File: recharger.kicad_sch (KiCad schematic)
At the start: 20 parts, among them J1 Battery Connector, U2 BQ25887RGE

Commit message: update PCB
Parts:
- J1: footprint Connector_JST:JST_PH_S4B-PH-K_1x04_P2.00mm_Horizontal -> Connector_JST:JST_PH_S4B-PH-SM4-TB_1x04-1MP_P2.00mm_Horizontal
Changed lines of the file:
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@@
 			)
 		)
-		(property "Footprint" "Connector_JST:JST_PH_S4B-PH-K_1x04_P2.00mm_Horizontal"
+		(property "Footprint" "Connector_JST:JST_PH_S4B-PH-SM4-TB_1x04-1MP_P2.00mm_Horizontal"
 			(at 194.31 110.49 0)
 			(hide yes)

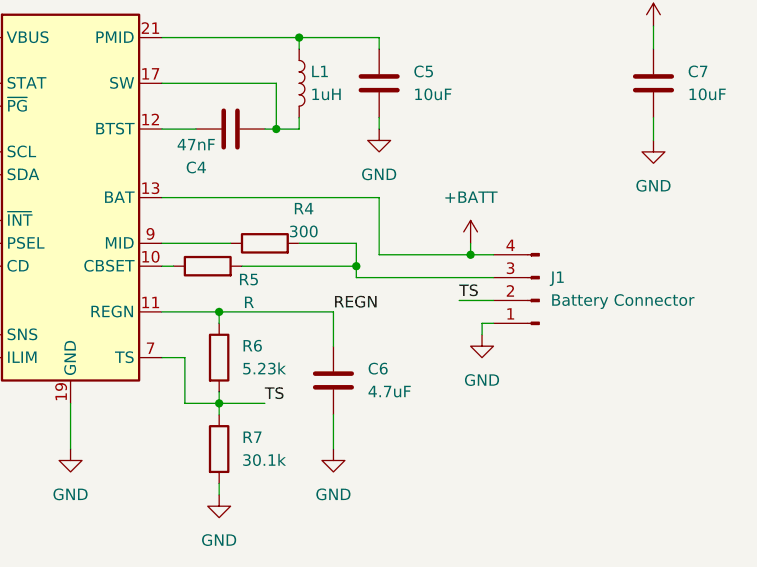
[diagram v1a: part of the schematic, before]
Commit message: more on layout
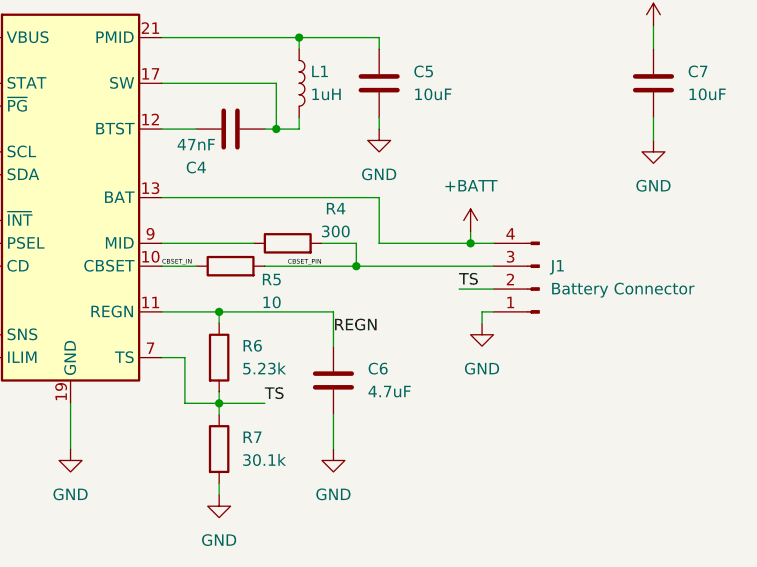
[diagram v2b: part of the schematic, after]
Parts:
- R5: value R -> 10
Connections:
- net CBSET_PIN: now reaches J1.3 (Pin_3), R4.2, R5.2
- net CBSET_IN: now reaches R5.1, U2.10 (CBSET)
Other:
- moved on the sheet: J1, R4, R5
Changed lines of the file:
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@@
 	)
 	(junction
-		(at 186.69 105.41)
+		(at 186.69 104.14)
 		(diameter 0)
 		(color 0 0 0 0)
@@
 	)
 	(junction
-		(at 173.99 106.68)
+		(at 158.75 121.92)
 		(diameter 0)
 		(color 0 0 0 0)
@@
 	)
 	(junction
-		(at 158.75 121.92)
+		(at 173.99 106.68)
 		(diameter 0)
 		(color 0 0 0 0)
@@
 	(wire
 		(pts
-			(xy 186.69 104.14) (xy 186.69 105.41)
+			(xy 186.69 102.87) (xy 186.69 104.14)
 		)
 		(stroke
@@
 	(wire
 		(pts
-			(xy 176.53 99.06) (xy 176.53 105.41)
+			(xy 176.53 99.06) (xy 176.53 104.14)
 		)
 		(stroke
@@
 	(wire
 		(pts
-			(xy 161.29 106.68) (xy 173.99 106.68)
+			(xy 163.83 106.68) (xy 173.99 106.68)
 		)
 		(stroke
@@
 	(wire
 		(pts
-			(xy 185.42 110.49) (xy 189.23 110.49)
+			(xy 185.42 109.22) (xy 189.23 109.22)
 		)
 		(stroke
@@
 	(wire
 		(pts
-			(xy 173.99 104.14) (xy 167.64 104.14)
+			(xy 173.99 104.14) (xy 170.18 104.14)
 		)
 		(stroke
@@
 	(wire
 		(pts
-			(xy 187.96 113.03) (xy 189.23 113.03)
+			(xy 187.96 111.76) (xy 189.23 111.76)
 		)
 		(stroke
@@
 	(wire
 		(pts
-			(xy 173.99 107.95) (xy 189.23 107.95)
+			(xy 173.99 106.68) (xy 189.23 106.68)
 		)
 		(stroke
@@
 	(wire
 		(pts
-			(xy 187.96 113.03) (xy 187.96 114.3)
+			(xy 187.96 111.76) (xy 187.96 113.03)
 		)
 		(stroke
@@
 	(wire
 		(pts
-			(xy 152.4 106.68) (xy 153.67 106.68)
+			(xy 152.4 106.68) (xy 156.21 106.68)
 		)
 		(stroke
@@
 	(wire
 		(pts
-			(xy 186.69 105.41) (xy 189.23 105.41)
+			(xy 186.69 104.14) (xy 189.23 104.14)
 		)
 		(stroke
@@
 	(wire
 		(pts
-			(xy 152.4 104.14) (xy 160.02 104.14)
+			(xy 152.4 104.14) (xy 162.56 104.14)
 		)
 		(stroke
@@
 	(wire
 		(pts
-			(xy 176.53 105.41) (xy 186.69 105.41)
+			(xy 176.53 104.14) (xy 186.69 104.14)
 		)
 		(stroke
@@
 	(wire
 		(pts
-			(xy 173.99 106.68) (xy 173.99 107.95)
-		)
-		(stroke
-			(width 0)
-			(type default)
-		)
-	)
-	(wire
-		(pts
 			(xy 127 106.68) (xy 132.08 106.68)
 		)
@@
 		)
 	)
+	(label "CBSET_IN"
+		(at 152.4 106.68 0)
+		(effects
+			(font
+				(size 0.508 0.508)
+			)
+			(justify left bottom)
+		)
+	)
 	(label "SCL"
 		(at 118.11 93.98 0)
@@
 		)
 	)
+	(label "CBSET_PIN"
+		(at 166.37 106.68 0)
+		(effects
+			(font
+				(size 0.508 0.508)
+			)
+			(justify left bottom)
+		)
+	)
 	(label "REGN"
 		(at 119.38 67.31 0)
@@
 	)
 	(label "TS"
-		(at 185.42 110.49 0)
+		(at 185.42 109.22 0)
 		(effects
 			(font
@@
 	)
 	(label "REGN"
-		(at 171.45 111.76 0)
+		(at 171.45 114.3 0)
 		(effects
 			(font
@@
 	(symbol
 		(lib_id "Connector:Conn_01x04_Pin")
-		(at 194.31 110.49 180)
+		(at 194.31 109.22 180)
 		(unit 1)
 		(body_style 1)
@@
 		(fields_autoplaced yes)
 		(property "Reference" "J1"
-			(at 195.58 107.9499 0)
+			(at 195.58 106.6799 0)
 			(show_name no)
 			(do_not_autoplace no)
@@
 		)
 		(property "Value" "Battery Connector"
-			(at 195.58 110.4899 0)
+			(at 195.58 109.2199 0)
 			(show_name no)
 			(do_not_autoplace no)
@@
 		)
 		(property "Footprint" "Connector_JST:JST_PH_S4B-PH-SM4-TB_1x04-1MP_P2.00mm_Horizontal"
-			(at 194.31 110.49 0)
+			(at 194.31 109.22 0)
 			(hide yes)
 			(show_name no)
@@
 		)
 		(property "Datasheet" ""
-			(at 194.31 110.49 0)
+			(at 194.31 109.22 0)
 			(hide yes)
 			(show_name no)
@@
 		)
 		(property "Description" "Generic connector, single row, 01x04, script generated"
-			(at 194.31 110.49 0)
+			(at 194.31 109.22 0)
 			(hide yes)
 			(show_name no)
@@
 	(symbol
 		(lib_id "power:GND")
-		(at 187.96 114.3 0)
+		(at 187.96 113.03 0)
 		(unit 1)
 		(body_style 1)
@@
 		(fields_autoplaced yes)
 		(property "Reference" "#PWR015"
-			(at 187.96 120.65 0)
+			(at 187.96 119.38 0)
 			(hide yes)
 			(show_name no)
@@
 		)
 		(property "Value" "GND"
-			(at 187.96 119.38 0)
+			(at 187.96 118.11 0)
 			(show_name no)
 			(do_not_autoplace no)
@@
 		)
 		(property "Footprint" ""
-			(at 187.96 114.3 0)
+			(at 187.96 113.03 0)
 			(hide yes)
 			(show_name no)
@@
 		)
 		(property "Datasheet" ""
-			(at 187.96 114.3 0)
+			(at 187.96 113.03 0)
 			(hide yes)
 			(show_name no)
@@
 		)
 		(property "Description" "Power symbol creates a global label with name \"GND\" , ground"
-			(at 187.96 114.3 0)
+			(at 187.96 113.03 0)
 			(hide yes)
 			(show_name no)
@@
 	(symbol
 		(lib_id "power:+BATT")
-		(at 186.69 104.14 0)
+		(at 186.69 102.87 0)
 		(unit 1)
 		(body_style 1)
@@
 		(fields_autoplaced yes)
 		(property "Reference" "#PWR018"
-			(at 186.69 107.95 0)
+			(at 186.69 106.68 0)
 			(hide yes)
 			(show_name no)
@@
 		)
 		(property "Value" "+BATT"
-			(at 186.69 99.06 0)
+			(at 186.69 97.79 0)
 			(show_name no)
 			(do_not_autoplace no)
@@
 		)
 		(property "Footprint" ""
-			(at 186.69 104.14 0)
+			(at 186.69 102.87 0)
 			(hide yes)
 			(show_name no)
@@
 		)
 		(property "Datasheet" ""
-			(at 186.69 104.14 0)
+			(at 186.69 102.87 0)
 			(hide yes)
 			(show_name no)
@@
 		)
 		(property "Description" "Power symbol creates a global label with name \"+BATT\""
-			(at 186.69 104.14 0)
+			(at 186.69 102.87 0)
 			(hide yes)
 			(show_name no)
@@
 	(symbol
 		(lib_id "Device:R")
-		(at 157.48 106.68 90)
+		(at 160.02 106.68 90)
 		(unit 1)
 		(body_style 1)
@@
 		(dnp no)
 		(property "Reference" "R5"
-			(at 162.052 108.204 90)
+			(at 164.592 108.204 90)
 			(show_name no)
 			(do_not_autoplace no)
@@
 			)
 		)
-		(property "Value" "R"
-			(at 162.052 110.744 90)
+		(property "Value" "10"
+			(at 164.592 110.744 90)
 			(show_name no)
 			(do_not_autoplace no)
@@
 		)
 		(property "Footprint" "Resistor_SMD:R_2512_6332Metric"
-			(at 157.48 108.458 90)
+			(at 160.02 108.458 90)
 			(hide yes)
 			(show_name no)
@@
 		)
 		(property "Datasheet" ""
-			(at 157.48 106.68 0)
+			(at 160.02 106.68 0)
 			(hide yes)
 			(show_name no)
@@
 		)
 		(property "Description" "Resistor"
-			(at 157.48 106.68 0)
+			(at 160.02 106.68 0)
 			(hide yes)
 			(show_name no)
@@
 	(symbol
 		(lib_id "Device:R")
-		(at 163.83 104.14 90)
+		(at 166.37 104.14 90)
 		(unit 1)
 		(body_style 1)
@@
 		(dnp no)
 		(property "Reference" "R4"
-			(at 168.148 100.33 90)
+			(at 171.704 100.33 90)
 			(show_name no)
 			(do_not_autoplace no)
@@
 		)
 		(property "Value" "300"
-			(at 168.148 102.87 90)
+			(at 171.704 102.87 90)
 			(show_name no)
 			(do_not_autoplace no)
@@
 		)
 		(property "Footprint" "Resistor_SMD:R_0603_1608Metric"
-			(at 163.83 105.918 90)
+			(at 166.37 105.918 90)
 			(hide yes)
 			(show_name no)
@@
 		)
 		(property "Datasheet" ""
-			(at 163.83 104.14 0)
+			(at 166.37 104.14 0)
 			(hide yes)
 			(show_name no)
@@
 		)
 		(property "Description" "Resistor"
-			(at 163.83 104.14 0)
+			(at 166.37 104.14 0)
 			(hide yes)
 			(show_name no)

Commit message: updates
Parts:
- L1: footprint Inductor_SMD:L_1008_2520Metric -> Inductor_SMD:L_Sunlord_MWSA0518S
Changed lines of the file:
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@@
 			)
 		)
-		(property "Footprint" "Inductor_SMD:L_1008_2520Metric"
+		(property "Footprint" "Inductor_SMD:L_Sunlord_MWSA0518S"
 			(at 167.64 86.36 0)
 			(hide yes)
